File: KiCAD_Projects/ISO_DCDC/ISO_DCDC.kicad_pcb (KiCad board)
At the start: 2 copper layers, 100 x 120 mm, 74 parts, among them IC1 PC817, IC2 PC817, IC3 PC817, IC4 PC817, IC5 PC817, P1 CONN_01X01, P10 CONN_01X02, P11 CONN_01X02, P12 CONN_01X01, P13 CONN_01X04, P14 CONN_01X02, P15 CONN_01X02, P16 CONN_01X02, P19 CONN_01X01, P2 CONN_01X01, P20 CONN_01X01, P21 CONN_01X02, P22 CONN_01X01, P23 CONN_01X01, P25 CONN_01X01, P26 CONN_01X01, P3 CONN_01X01, P30 CONN_01X01, P4 CONN_01X02, P5 CONN_01X02, P6 CONN_01X04, P7 CONN_01X04, P8 CONN_01X01, P9 CONN_01X01, Q1 MOSFET_N, U1 V23076-D3001-D142, U2 V23076-D3001-D142, U3 V23076-D3001-D142

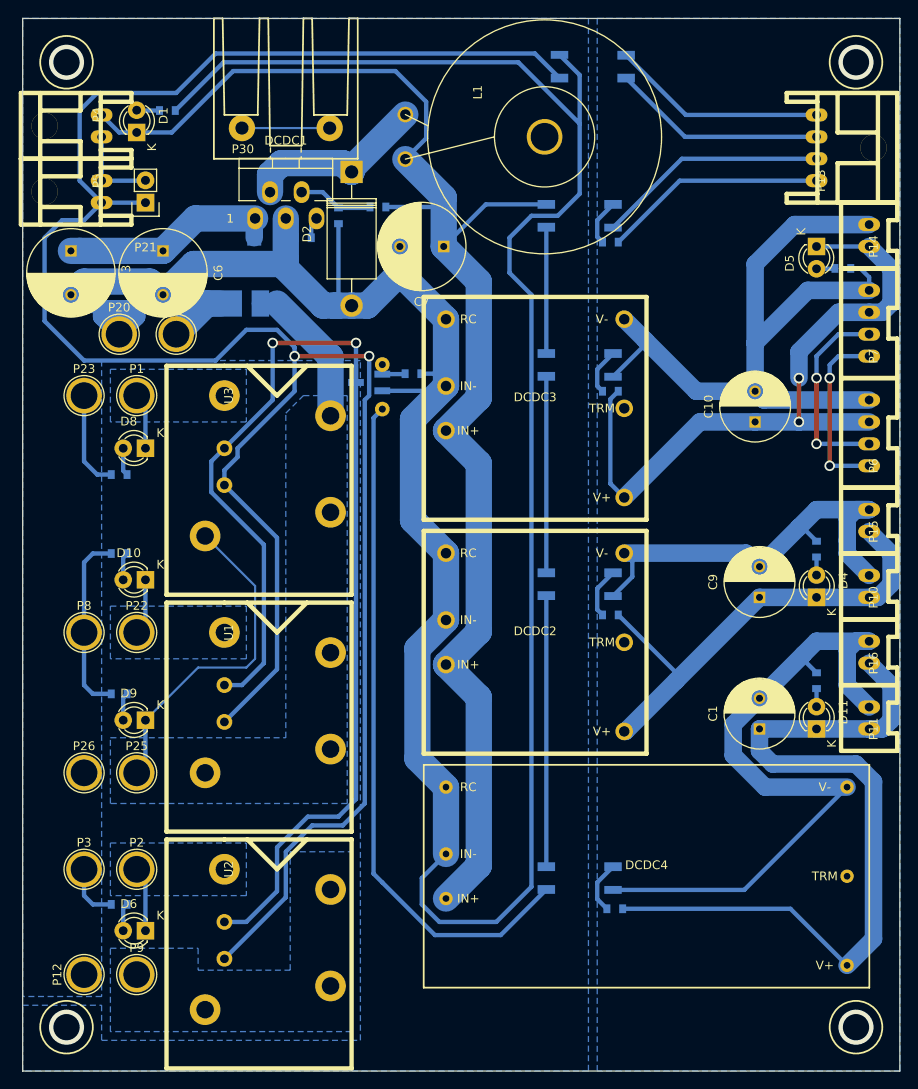
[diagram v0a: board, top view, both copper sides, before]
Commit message: no message
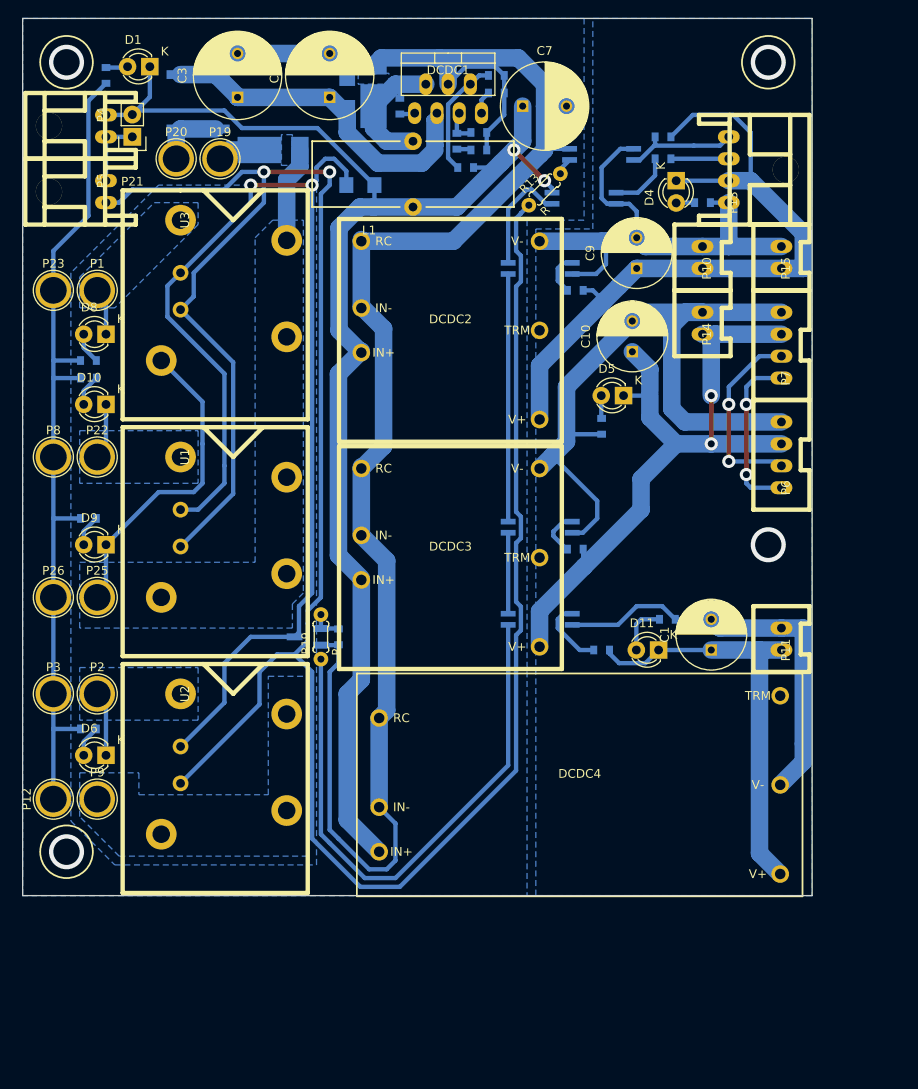
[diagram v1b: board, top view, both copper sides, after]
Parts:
- removed P16: CONN_01X02, RP_KiCAD_Connector:XA_2T
- removed P30: CONN_01X01, Heatsinks:16PB017_16.25.16
- added C11: 470p, RP_KiCAD_Libs:C1608_WP, B.Cu at (52.0, 15.0)
- added C2: 0.22u, RP_KiCAD_Libs:C1608_WP, B.Cu at (43.0, 10.0)
- added C8: 470p, RP_KiCAD_Libs:C1608_WP, B.Cu at (52.0, 13.0)
- added D7: DIODE, RP_KiCAD_Libs:C3216, B.Cu at (38.5, 19.0)
- added R10: 100k, RP_KiCAD_Libs:C1608_WP, B.Cu at (49.5, 14.0)
- added R13: R, RP_KiCAD_Libs:0204_2f5, F.Cu at (59.5, 19.5)
- added R14: R, RP_KiCAD_Libs:C1608_WP, B.Cu at (73.0, 13.5)
- D2: footprint Diodes_ThroughHole:Diode_DO-201AD_Horizontal_RM15 -> Diodes_SMD:POWER_DI5; moved to B.Cu
- DCDC1: value SI-8008HFE -> SI-8010Y; footprint TO_SOT_Packages_THT:Pentawatt_Neutral_Staggered_Verical_TO220-5-T05D -> TO_SOT_Packages_THT:TO-220_7_Vertical
- IC1, IC2, IC3, IC4, IC5: footprint Opto-Devices:Optocoupler_SMD_HandSoldering_KPC357_LTV35x_PC357_SingleChannel -> Housings_SOIC:SOIJ-4_5.3x5.3mm_Pitch1.27mm
- L1: footprint Choke_Toroid_ThroughHole:Choke_Toroid_horizontal_Diameter26mm -> Choke_Toroid_ThroughHole:Choke_Toroid_8.5x24mm_Vertical
- R19: moved to F.Cu
- R3: value R -> 15k
- R4: value R -> 1k
- moved D4 50.1 mm to (74.5, 18.5), turned to 270 degrees
- moved P10 42.0 mm to (77.5, 28.5)
- moved R7 41.6 mm to (77.5, 21.0), turned to 0 degrees
- moved C9 40.0 mm to (70.0, 28.5)
- moved DCDC2 36.8 mm to (48.8, 35.6)
- moved R8 32.9 mm to (66.0, 46.5), turned to 270 degrees
- moved P15 31.6 mm to (86.5, 28.5)
- moved R11 31.2 mm to (36.0, 70.5), turned to 270 degrees
- moved IC3 29.8 mm to (59.0, 68.5)
- moved Q1 29.8 mm to (32.5, 70.5)
- moved R21 29.5 mm to (66.0, 72.0)
- moved R19 29.3 mm to (34.0, 70.5)
- moved D5 27.8 mm to (68.5, 43.0), turned to 180 degrees
- moved C5 27.5 mm to (54.0, 8.50), turned to 180 degrees
- moved C3 25.8 mm to (24.5, 9.00), turned to 90 degrees
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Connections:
- DCDC1 pad 1: Net-(C3-Pad1) -> Net-(C2-Pad2)
- DCDC1 pad 3: GNDPWR -> Net-(C3-Pad1)
- DCDC1 pad 4: Net-(DCDC1-Pad4) -> GNDPWR
- DCDC1 pad 5: Net-(C5-Pad2) -> Net-(C8-Pad1)
- IC1 pad 2: /12V_CAN_GND -> /5V_GND
- IC2 pad 2: /5V_GND -> /12V_CAN_GND
- IC4 pad 2: Net-(IC4-Pad2) -> /5V_GND
- IC5 pad 1: /POWER_EN_HIGH -> Net-(IC5-Pad1)
- IC5 pad 3: Net-(IC5-Pad3) -> /5V_GND
- P13 pad 1: Net-(P13-Pad1) -> /5V_GND
- P13 pad 2: Net-(IC4-Pad2) -> /5V
- P13 pad 3: Net-(IC5-Pad4) -> Net-(P13-Pad3)
- P13 pad 4: Net-(IC5-Pad3) -> Net-(IC5-Pad4)
- P21 pad 1: /POWER_EN_HIGH -> Net-(P21-Pad1)
- P21 pad 2: Net-(P21-Pad2) -> /15V
- P4 pad 2: Net-(P21-Pad2) -> Net-(P21-Pad1)
- P5 pad 1: Net-(P21-Pad2) -> Net-(P21-Pad1)
- R22 pad 1: Net-(P13-Pad1) -> Net-(P13-Pad3)
- R3 pad 1: Net-(DCDC1-Pad4) -> Net-(DCDC1-Pad6)
- R4 pad 2: Net-(DCDC1-Pad4) -> Net-(DCDC1-Pad6)
- R6 pad 1: /5V -> /12V_CAN
- R9 pad 1: /12V_CAN -> /5V
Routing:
- net GNDPWR: track 362.4 -> 301.6 mm
- net /12V_RasPi: track 90.4 -> 47.6 mm
- net /12V_RasPi_GND: track 82.8 -> 47.2 mm
- net Net-(IC4-Pad2): track 26.5 -> 0.00 mm
- net /5V: track 55.3 -> 81.1 mm
- net Net-(P13-Pad1): track 25.5 -> 0.00 mm
- net Net-(IC5-Pad3): track 24.5 -> 0.00 mm
- net Net-(IC2-Pad3): track 30.9 -> 9.23 mm
- net Net-(C3-Pad1): track 30.7 -> 49.9 mm
- net +BATT: track 64.0 -> 47.2 mm
- net Net-(DCDC1-Pad6): track 0.00 -> 13.9 mm
- net Net-(IC3-Pad3): track 78.1 -> 64.7 mm
- net /POWER_EN_HIGH: track 262.5 -> 275.7 mm
- net Net-(IC5-Pad4): track 24.5 -> 13.0 mm
- net /12V_CAN: track 78.9 -> 89.8 mm
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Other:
- board size 100 x 120 mm -> 90 x 100 mm
